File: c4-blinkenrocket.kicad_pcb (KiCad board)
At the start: 2 copper layers, 47 x 96.3 mm, 26 parts, among them J1 ISP, SW1 SW_SPST, SW2 SW_SPST, U1 ATtiny88-AU, U2 24CW640-I_SN

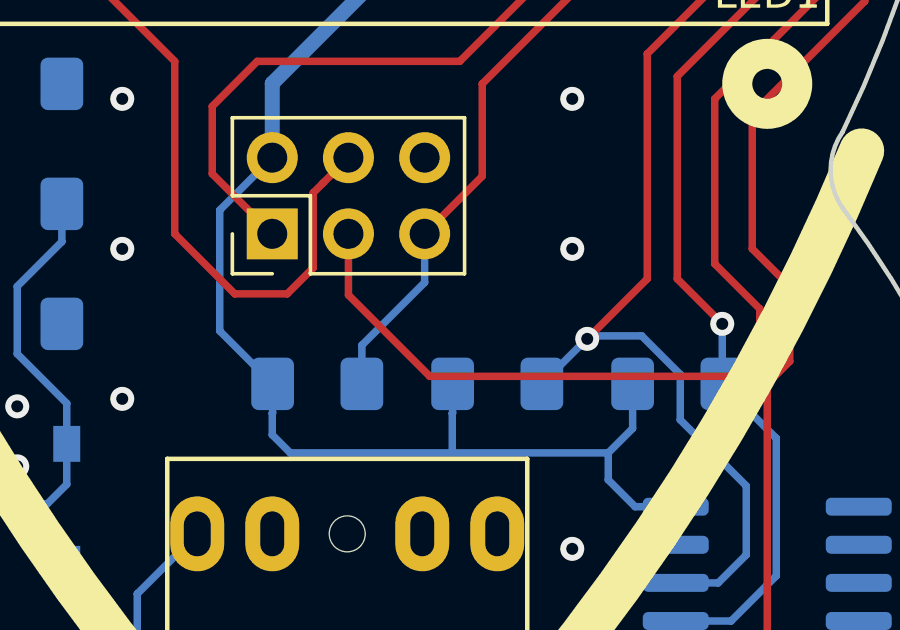
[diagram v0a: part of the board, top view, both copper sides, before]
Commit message: Fabrication data as ordered at the usual chinese pcb manufactures
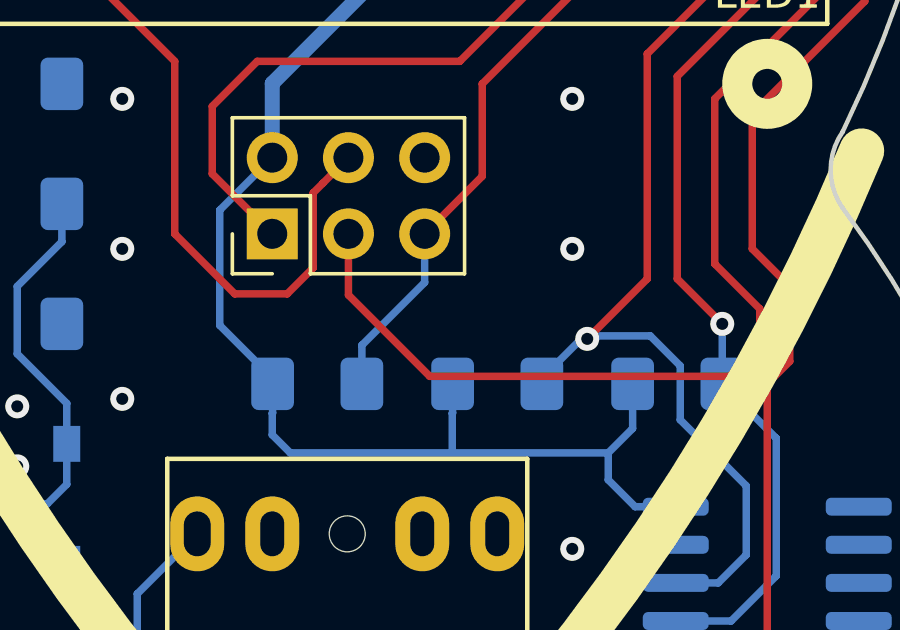
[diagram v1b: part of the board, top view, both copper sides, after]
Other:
- rule pad_to_mask_clearance: 0.051 -> 0.05
- rule solder_mask_min_width: 0.25 -> 0.15
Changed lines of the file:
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@@
     (thickness 1.6)
     (drawings 38)
-    (tracks 413)
+    (tracks 415)
     (zones 0)
     (modules 26)
@@
   )
   (setup
-    (last_trace_width 0.5)
+    (last_trace_width 0.25)
     (user_trace_width 0.25)
     (user_trace_width 0.4)
@@
     (pad_size 1.524 1.524)
     (pad_drill 0.762)
-    (pad_to_mask_clearance 0.051)
-    (solder_mask_min_width 0.25)
+    (pad_to_mask_clearance 0.05)
+    (solder_mask_min_width 0.15)
+    (pad_to_paste_clearance_ratio -0.1)
     (aux_axis_origin 100 150)
     (grid_origin 100 150)
     (visible_elements FFFFFF7F)
     (pcbplotparams
-      (layerselection 0x010fc_ffffffff)
-      (usegerberextensions false)
-      (usegerberattributes false)
+      (layerselection 0x010f4_ffffffff)
+      (usegerberextensions true)
+      (usegerberattributes true)
       (usegerberadvancedattributes false)
       (creategerberjobfile false)
-      (excludeedgelayer true)
-      (linewidth 0.100000)
+      (excludeedgelayer false)
+      (linewidth 0.150000)
       (plotframeref false)
       (viasonmask false)
       (mode 1)
-      (useauxorigin false)
+      (useauxorigin true)
       (hpglpennumber 1)
       (hpglpenspeed 20)
@@
       (outputformat 1)
       (mirror false)
-      (drillshape 1)
+      (drillshape 0)
       (scaleselection 1)
-      (outputdirectory ""))
+      (outputdirectory "fab/"))
   )
   (net 0 "")
@@
     (descr "Capacitor SMD 1206 (3216 Metric), square (rectangular) end terminal, IPC_7351 nominal with elongated pad for handsoldering. (Body size source: http://www.tortai-tech.com/upload/download/2011102023233369053.pdf), generated with kicad-footprint-generator")
     (tags "capacitor handsolder")
+    (solder_paste_margin -10)
     (attr smd)
     (fp_text reference C3 (at 0 1.82) (layer B.SilkS)
@@
     (descr "Resistor SMD 1206 (3216 Metric), square (rectangular) end terminal, IPC_7351 nominal with elongated pad for handsoldering. (Body size source: http://www.tortai-tech.com/upload/download/2011102023233369053.pdf), generated with kicad-footprint-generator")
     (tags "resistor handsolder")
+    (solder_paste_margin -10)
     (attr smd)
     (fp_text reference R6 (at 0 1.82) (layer B.SilkS)
@@
     (descr "Resistor SMD 1206 (3216 Metric), square (rectangular) end terminal, IPC_7351 nominal with elongated pad for handsoldering. (Body size source: http://www.tortai-tech.com/upload/download/2011102023233369053.pdf), generated with kicad-footprint-generator")
     (tags "resistor handsolder")
+    (solder_paste_margin -10)
     (attr smd)
     (fp_text reference R5 (at 0 -2 180) (layer B.SilkS)
@@
     (descr "Resistor SMD 1206 (3216 Metric), square (rectangular) end terminal, IPC_7351 nominal with elongated pad for handsoldering. (Body size source: http://www.tortai-tech.com/upload/download/2011102023233369053.pdf), generated with kicad-footprint-generator")
     (tags "resistor handsolder")
+    (solder_paste_margin -10)
     (attr smd)
     (fp_text reference R4 (at 0 -2 180) (layer B.SilkS)
@@
     (descr "Resistor SMD 1206 (3216 Metric), square (rectangular) end terminal, IPC_7351 nominal with elongated pad for handsoldering. (Body size source: http://www.tortai-tech.com/upload/download/2011102023233369053.pdf), generated with kicad-footprint-generator")
     (tags "resistor handsolder")
+    (solder_paste_margin -10)
     (attr smd)
     (fp_text reference R3 (at 0 1.9) (layer B.SilkS)
@@
     (descr "Resistor SMD 1206 (3216 Metric), square (rectangular) end terminal, IPC_7351 nominal with elongated pad for handsoldering. (Body size source: http://www.tortai-tech.com/upload/download/2011102023233369053.pdf), generated with kicad-footprint-generator")
     (tags "resistor handsolder")
+    (solder_paste_margin -10)
     (attr smd)
     (fp_text reference R2 (at 0 -2 180) (layer B.SilkS)
@@
     (descr "Resistor SMD 1206 (3216 Metric), square (rectangular) end terminal, IPC_7351 nominal with elongated pad for handsoldering. (Body size source: http://www.tortai-tech.com/upload/download/2011102023233369053.pdf), generated with kicad-footprint-generator")
     (tags "resistor handsolder")
+    (solder_paste_margin -10)
     (attr smd)
     (fp_text reference R1 (at 0 2) (layer B.SilkS)
@@
     (descr "Capacitor SMD 1206 (3216 Metric), square (rectangular) end terminal, IPC_7351 nominal with elongated pad for handsoldering. (Body size source: http://www.tortai-tech.com/upload/download/2011102023233369053.pdf), generated with kicad-footprint-generator")
     (tags "capacitor handsolder")
+    (solder_paste_margin -10)
     (attr smd)
     (fp_text reference C2 (at 0 -2 180) (layer B.SilkS)
@@
     (descr "Capacitor SMD 1206 (3216 Metric), square (rectangular) end terminal, IPC_7351 nominal with elongated pad for handsoldering. (Body size source: http://www.tortai-tech.com/upload/download/2011102023233369053.pdf), generated with kicad-footprint-generator")
     (tags "capacitor handsolder")
+    (solder_paste_margin -10)
     (attr smd)
     (fp_text reference C1 (at 0 1.82) (layer B.SilkS)
@@
     (descr SOD-123)
     (tags SOD-123)
+    (solder_paste_margin -10)
     (attr smd)
     (fp_text reference D2 (at 0 2) (layer B.SilkS)
@@
     (descr SOD-123)
     (tags SOD-123)
+    (solder_paste_margin -10)
     (attr smd)
     (fp_text reference D1 (at 0 2) (layer B.SilkS)
@@
   (segment (start 126.4875 103) (end 126.4875 101.7375) (width 0.4) (layer B.Cu) (net 3))
   (segment (start 126.4875 101.7375) (end 125.4 100.65) (width 0.4) (layer B.Cu) (net 3))
-  (segment (start 120.75 111.21) (end 122.5 109.46) (width 0.25) (layer B.Cu) (net 3))
-  (segment (start 122.5125 117) (end 120.75 115.2375) (width 0.25) (layer B.Cu) (net 3))
-  (segment (start 120.75 115.2375) (end 120.75 111.21) (width 0.25) (layer B.Cu) (net 3))
   (segment (start 114.6 72.5) (end 114.6 69.5) (width 0.5) (layer B.Cu) (net 3))
   (segment (start 109.6 77.5) (end 114.6 72.5) (width 0.5) (layer B.Cu) (net 3))
@@
   (segment (start 114.6 72.5) (end 114.6 72.6) (width 0.5) (layer F.Cu) (net 3))
   (segment (start 114.6 72.6) (end 117 75) (width 0.5) (layer F.Cu) (net 3))
+  (segment (start 120.75 111.21) (end 122.5 109.46) (width 0.25) (layer B.Cu) (net 3))
+  (segment (start 120.75 115.05) (end 120.75 111.21) (width 0.25) (layer B.Cu) (net 3))
+  (segment (start 122.5125 117) (end 122.5125 116.8125) (width 0.25) (layer B.Cu) (net 3))
+  (segment (start 122.5125 116.8125) (end 120.75 115.05) (width 0.25) (layer B.Cu) (net 3))
   (segment (start 112.5125 114.025) (end 112.5125 111) (width 0.25) (layer B.Cu) (net 4))
   (segment (start 112.5125 115) (end 112.5125 114.025) (width 0.25) (layer B.Cu) (net 4))
@@
   (segment (start 111.774999 94.761999) (end 112.411999 94.124999) (width 0.25) (layer B.Cu) (net 33))
   (segment (start 115.024999 94.124999) (end 116.1 95.2) (width 0.25) (layer B.Cu) (net 33))
-  (segment (start 137.365 123.635) (end 136.3 123.635) (width 0.25) (layer B.Cu) (net 34))
-  (segment (start 138.3 122.7) (end 137.365 123.635) (width 0.25) (layer B.Cu) (net 34))
-  (segment (start 138.3 120.4) (end 138.3 122.7) (width 0.25) (layer B.Cu) (net 34))
-  (segment (start 133.0875 115.4) (end 134.81319 115.4) (width 0.25) (layer B.Cu) (net 34))
-  (segment (start 131.4875 117) (end 133.0875 115.4) (width 0.25) (layer B.Cu) (net 34))
-  (segment (start 136.1 116.68681) (end 136.1 118.2) (width 0.25) (layer B.Cu) (net 34))
-  (segment (start 134.81319 115.4) (end 136.1 116.68681) (width 0.25) (layer B.Cu) (net 34))
-  (segment (start 136.1 118.2) (end 138.3 120.4) (width 0.25) (layer B.Cu) (net 34))
   (via (at 133 115.5) (size 0.8) (drill 0.4) (layers F.Cu B.Cu) (net 34))
   (segment (start 134.785001 94.035001) (end 134.149999 93.399999) (width 0.25) (layer F.Cu) (net 34))
@@
   (segment (start 139.5 101.5) (end 139.5 95) (width 0.25) (layer F.Cu) (net 34))
   (segment (start 133.350001 93.399999) (end 133.75 93) (width 0.25) (layer B.Cu) (net 34))
+  (segment (start 137.365 123.635) (end 136.3 123.635) (width 0.25) (layer B.Cu) (net 34))
+  (segment (start 136.1 118.2) (end 138.3 120.4) (width 0.25) (layer B.Cu) (net 34))
+  (segment (start 131.4875 117) (end 131.4875 116.8125) (width 0.25) (layer B.Cu) (net 34))
+  (segment (start 131.4875 116.8125) (end 132.9 115.4) (width 0.25) (layer B.Cu) (net 34))
+  (segment (start 132.9 115.4) (end 135.1 115.4) (width 0.25) (layer B.Cu) (net 34))
+  (segment (start 135.1 115.4) (end 136.1 116.4) (width 0.25) (layer B.Cu) (net 34))
+  (segment (start 138.3 122.7) (end 137.365 123.635) (width 0.25) (layer B.Cu) (net 34))
+  (segment (start 138.3 120.4) (end 138.3 122.7) (width 0.25) (layer B.Cu) (net 34))
+  (segment (start 136.1 116.4) (end 136.1 118.2) (width 0.25) (layer B.Cu) (net 34))
   (segment (start 139.3 118.8125) (end 137.4875 117) (width 0.25) (layer B.Cu) (net 35))
   (segment (start 139.3 123.4) (end 139.3 118.8125) (width 0.25) (layer B.Cu) (net 35))
